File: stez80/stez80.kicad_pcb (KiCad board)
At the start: 4 copper layers, 100 x 100 mm, 38 parts, among them J1 Conn_01x32_Pin, J2 Barrel_Jack, J3 DE9_Socket, SW1 SW_Push, U1 74HC14, U2 Z80CPU, U3 AS6C1008-xxP, U4 27C512, U5 ATmega16A-P, U6 Z80_SIO, U7 MAX232, Y1 CXO_DIP8

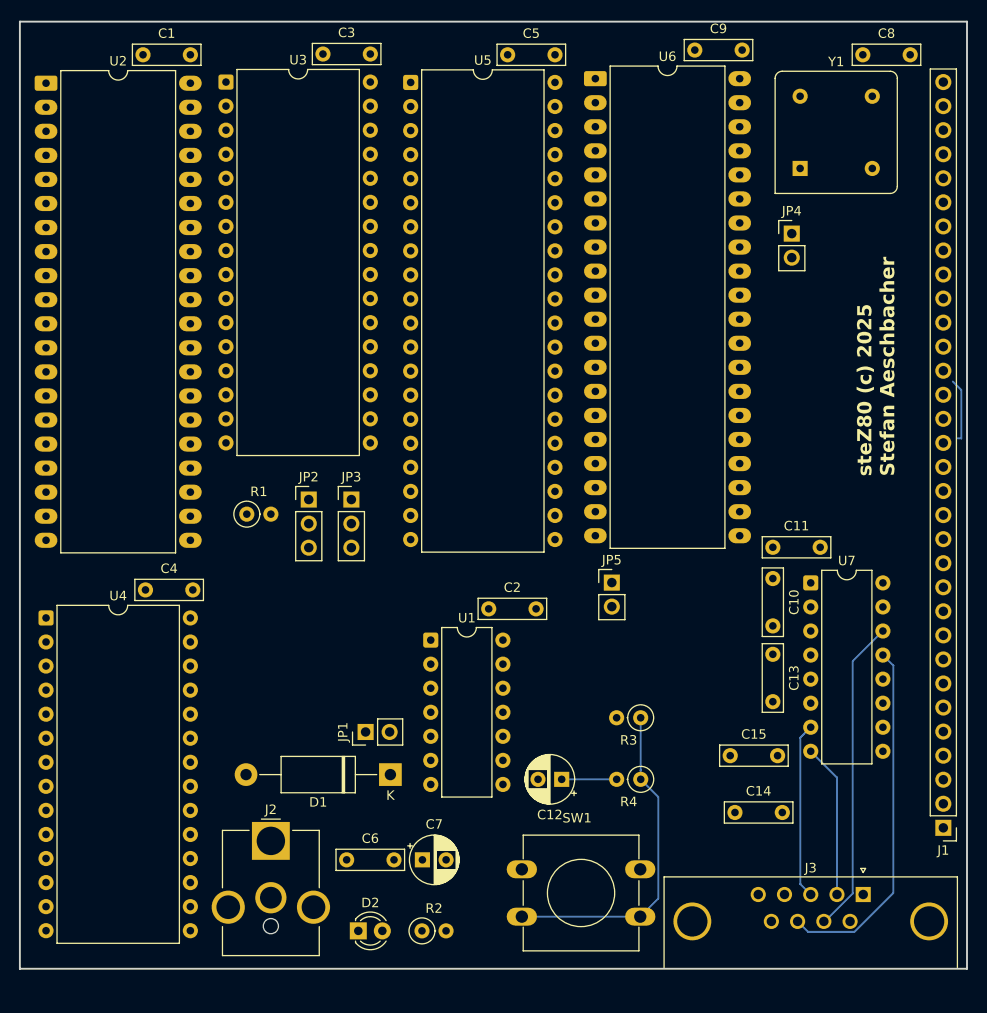
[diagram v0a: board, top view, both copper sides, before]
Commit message: pcb layout
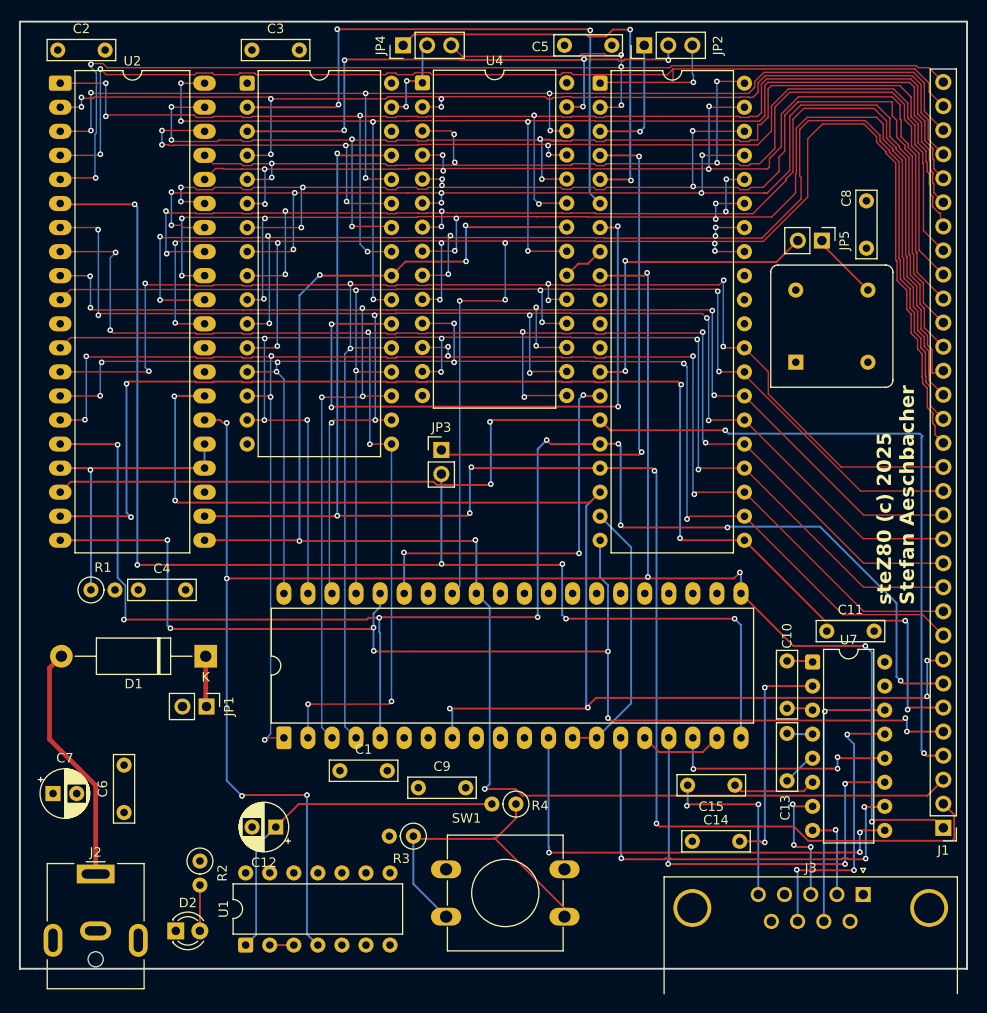
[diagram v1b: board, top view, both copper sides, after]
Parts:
- J2: footprint Connector_BarrelJack:BarrelJack_CUI_PJ-063AH_Horizontal_CircularHoles -> Connector_BarrelJack:BarrelJack_CUI_PJ-063AH_Horizontal
- J3: footprint Connector_Dsub:DSUB-9_Socket_Horizontal_P2.77x2.84mm_EdgePinOffset4.94mm_Housed_MountingHolesOffset4.94mm -> Connector_Dsub:DSUB-9_Socket_Horizontal_P2.77x2.84mm_EdgePinOffset7.70mm_Housed_MountingHolesOffset9.12mm
- moved C9 83.2 mm to (80.6, 104.4)
- moved C1 78.4 mm to (72.3, 102.6)
- moved U6 77.0 mm to (66.4, 99.1), turned to 90 degrees
- moved C2 74.5 mm to (42.5, 26.5)
- moved U4 69.1 mm to (81.0, 30.0)
- moved JP2 59.6 mm to (104.4, 26.0), turned to 90 degrees
- moved JP4 48.3 mm to (79.0, 26.0), turned to 90 degrees
- moved C7 39.6 mm to (42.0, 105.0)
- moved U1 37.7 mm to (62.3, 121.0), turned to 90 degrees
- moved C12 30.6 mm to (65.5, 108.5)
- moved R3 27.1 mm to (80.0, 109.5)
- moved R2 24.6 mm to (57.5, 112.1), turned to -90 degrees
- moved C6 24.0 mm to (49.5, 107.0), turned to 90 degrees
- moved D1 23.2 mm to (58.1, 90.5)
- moved JP3 22.8 mm to (83.0, 68.7)
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- renumbered JP5 to JP3, JP3 to JP4, JP4 to JP5
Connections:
- J1 pad 10: AddressBus14 -> Databus1
- J1 pad 11: AddressBus13 -> Databus2
- J1 pad 12: AddressBus12 -> Databus3
- J1 pad 13: AddressBus11 -> Databus4
- J1 pad 14: AddressBus10 -> Databus5
- J1 pad 15: AddressBus9 -> Databus6
- J1 pad 16: AddressBus8 -> Databus7
- J1 pad 17: AddressBus7 -> AddressBus0
- J1 pad 18: AddressBus6 -> AddressBus1
- J1 pad 19: AddressBus5 -> AddressBus2
- J1 pad 20: AddressBus4 -> AddressBus3
- J1 pad 21: AddressBus3 -> AddressBus4
- J1 pad 22: AddressBus2 -> AddressBus5
- J1 pad 23: AddressBus1 -> AddressBus6
- J1 pad 24: AddressBus0 -> AddressBus7
- J1 pad 25: Databus7 -> AddressBus8
- J1 pad 26: Databus6 -> AddressBus9
- J1 pad 27: Databus5 -> AddressBus10
- J1 pad 28: Databus4 -> AddressBus11
- J1 pad 29: Databus3 -> AddressBus12
- J1 pad 30: Databus2 -> AddressBus13
- J1 pad 31: Databus1 -> AddressBus14
- J1 pad 32: Databus0 -> AddressBus15
- J1 pad 9: AddressBus15 -> Databus0
- U2 pad 17: ~{NMI} -> Net-(U2-~{BUSRQ})
- U5 pad 33: AddressBus7 -> AddressBus0
- U5 pad 34: AddressBus6 -> AddressBus1
- U5 pad 35: AddressBus5 -> AddressBus2
- U5 pad 36: AddressBus4 -> AddressBus3
- U5 pad 37: AddressBus3 -> AddressBus4
- U5 pad 38: AddressBus2 -> AddressBus5
- U5 pad 39: AddressBus1 -> AddressBus6
- U5 pad 40: AddressBus0 -> AddressBus7
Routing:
- net ~{RESET}: track 0.00 -> 201.9 mm, vias 0 -> 9
- net AddressBus0: track 0.00 -> 198.4 mm, vias 0 -> 11
- net Databus3: track 0.00 -> 185.0 mm, vias 0 -> 10
- net Databus7: track 0.00 -> 174.4 mm, vias 0 -> 8
- net Databus5: track 0.00 -> 171.3 mm, vias 0 -> 9
- net ~{WR}: track 0.00 -> 170.4 mm, vias 0 -> 6
- net Databus1: track 0.00 -> 169.3 mm, vias 0 -> 9
- net ~{RD}: track 0.00 -> 164.8 mm, vias 0 -> 6
- net Databus4: track 0.00 -> 164.5 mm, vias 0 -> 9
- net ~{INT}: track 0.00 -> 162.6 mm, vias 0 -> 9
- net Databus0: track 0.00 -> 153.7 mm, vias 0 -> 8
- net AddressBus1: track 0.00 -> 153.1 mm, vias 0 -> 8
- net Databus2: track 0.00 -> 151.6 mm, vias 0 -> 7
- net Databus6: track 0.00 -> 149.7 mm, vias 0 -> 6
- net AddressBus2: track 0.00 -> 144.5 mm, vias 0 -> 8
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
